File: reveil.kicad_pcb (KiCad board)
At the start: 2 copper layers, 168.5 x 93 mm, 23 parts, among them Q1 2N3904, Q2 IRF540N, U1 MAX7219, U2 MAX7219

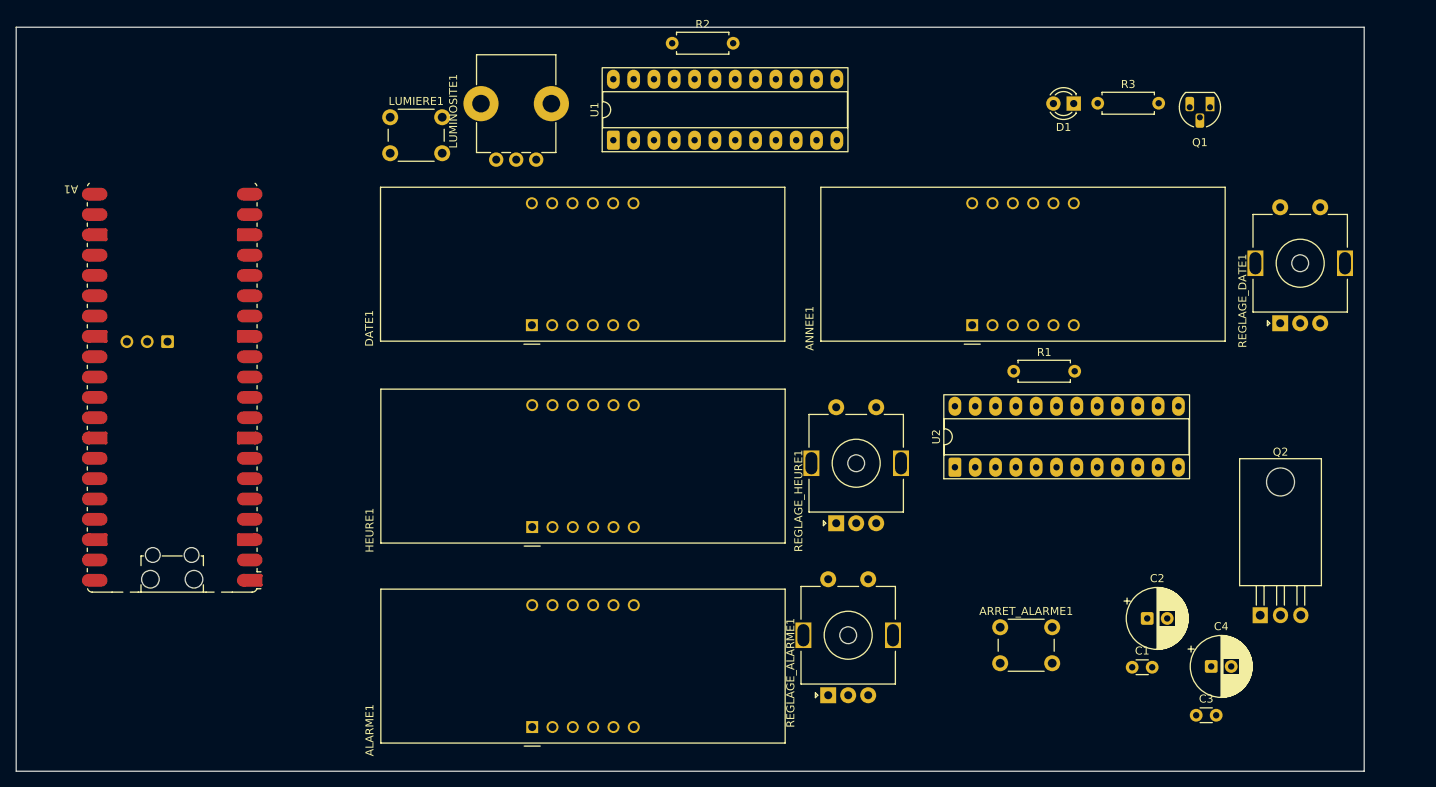
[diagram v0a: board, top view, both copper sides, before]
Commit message: contour du PCB
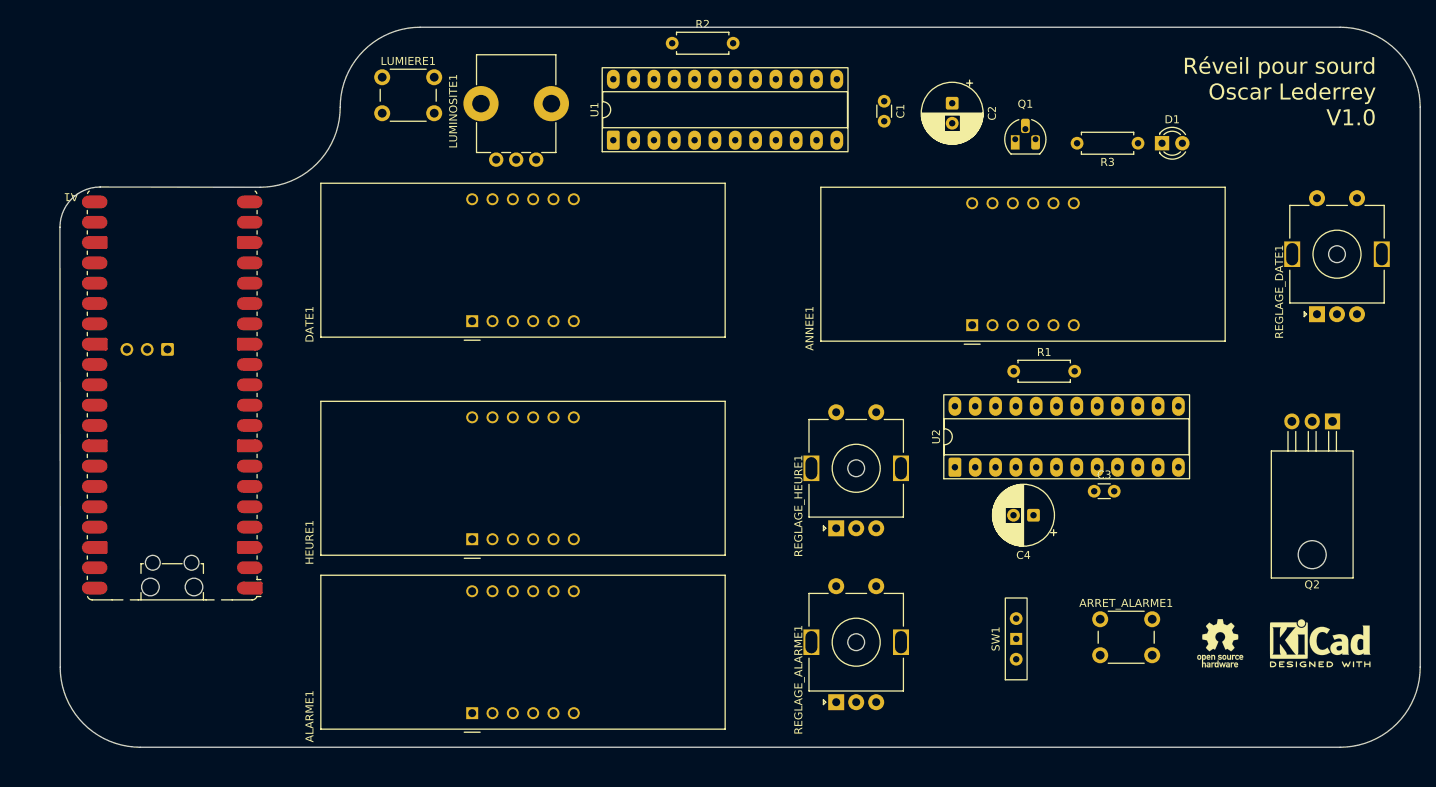
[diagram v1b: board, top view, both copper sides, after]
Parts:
- added REF**: OSHW-Logo_5.7x6mm_SilkScreen, Symbol:OSHW-Logo_5.7x6mm_SilkScreen, F.Cu at (225.0, 97.0)
- added REF**: KiCad-Logo2_5mm_SilkScreen, Symbol:KiCad-Logo2_5mm_SilkScreen, F.Cu at (237.5, 97.0)
- added SW1: SW_SPDT, Button_Switch_THT:SW_Slide-03_Wuerth-WS-SLTV_10x2.5x6.4_P2.54mm, F.Cu at (199.5, 96.5)
- moved C1 77.2 mm to (183.0, 29.2), turned to -90 degrees
- moved C2 68.9 mm to (191.5, 29.5), turned to -90 degrees
- moved C3 30.8 mm to (209.2, 78.0)
- moved C4 29.2 mm to (201.7, 81.0), turned to 180 degrees
- moved Q2 25.9 mm to (239.0, 69.3), turned to 180 degrees
- moved Q1 24.7 mm to (199.4, 34.0), turned to 0 degrees
- moved ARRET_ALARME1 12.5 mm to (210.0, 94.0)
- moved D1 12.1 mm to (217.7, 34.5), turned to 0 degrees
- moved ALARME1 7.70 mm to (131.5, 105.7)
- moved HEURE1 7.65 mm to (131.5, 84.0)
- moved DATE1 7.48 mm to (131.5, 56.7)
- moved R3 7.10 mm to (214.7, 34.5), turned to 180 degrees
- moved LUMIERE1 5.10 mm to (120.2, 26.2)
- moved REGLAGE_DATE1 4.74 mm to (237.1, 55.9)
- moved REGLAGE_ALARME1 1.33 mm to (177.0, 104.4)
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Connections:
- A1 pad 25: unconnected-(A1-GPIO19-Pad25) -> ALARME_ON_OFF
- U2 pad 19: VCC -> VBUS
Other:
- board size 168.5 x 93 mm -> 170 x 90 mm
- board text added: "Réveil pour sourd Oscar Lederrey V1.0"
